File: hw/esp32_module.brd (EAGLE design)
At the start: 61.6 x 53.3 mm, 2 parts, among them IC1 ESP32-S2_WROVER, IC2 ESP32-WROVER

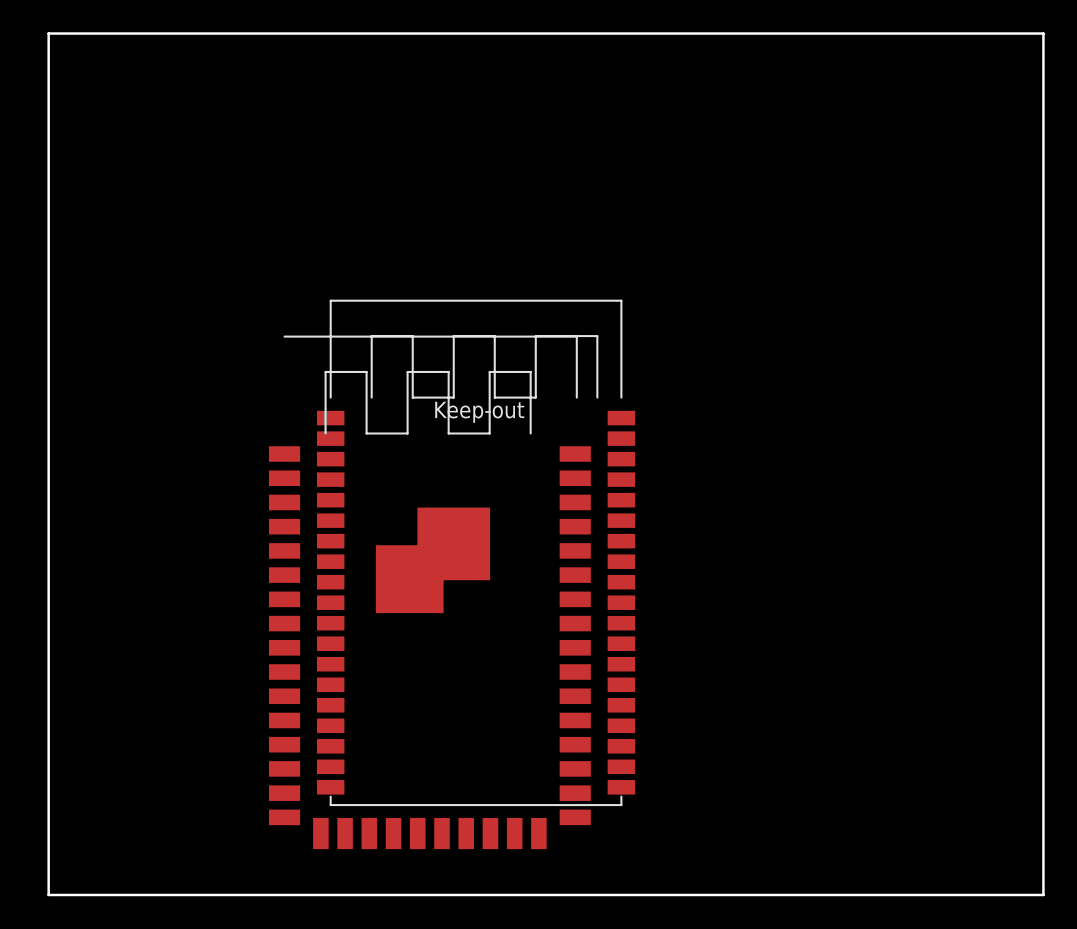
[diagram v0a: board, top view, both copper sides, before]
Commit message: improved
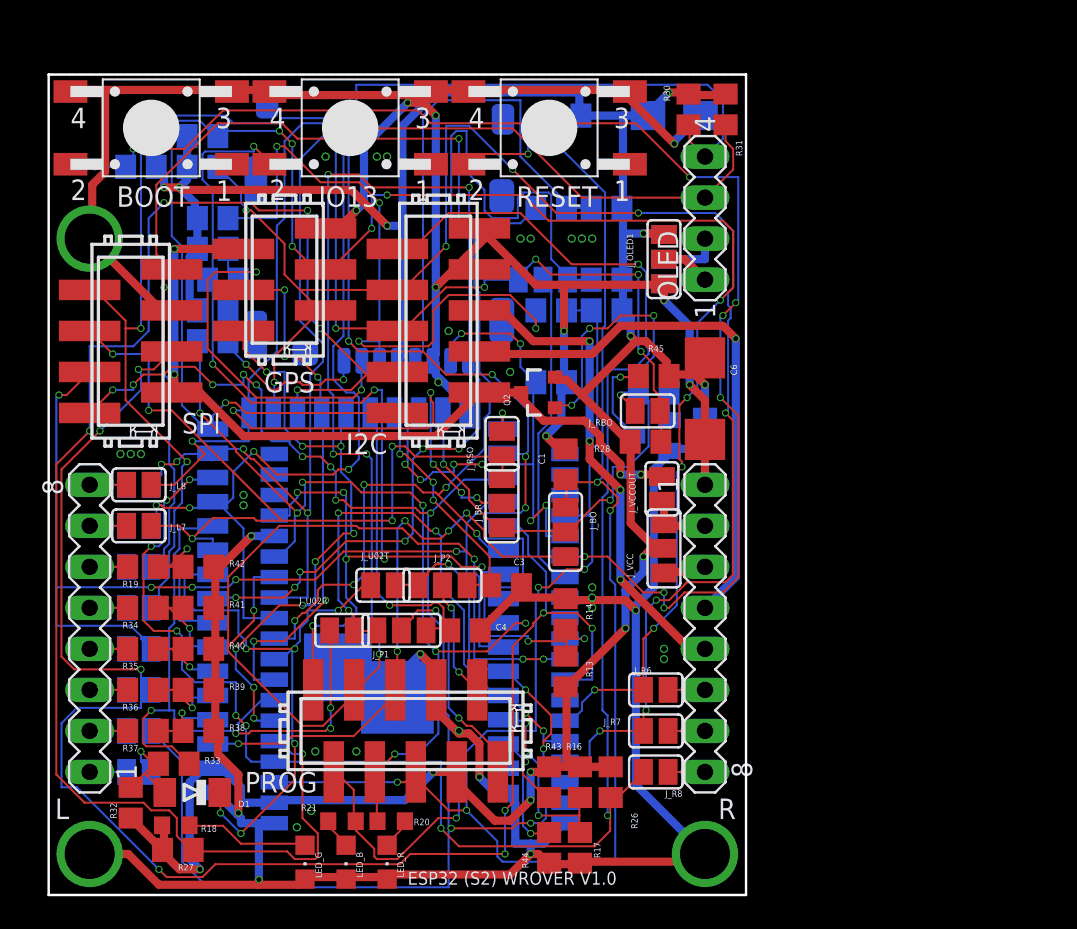
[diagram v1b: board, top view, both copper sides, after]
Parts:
- added BOOT, IO13, RESET: (no value), Ergaenzung:TASTER-9314_SMD
- added C1, C2: 0.1, rcl:C0805
- added C3, C4: 22p, rcl:C0805
- added C5: 10u, rcl:B/3528-21W
- added C6: (no value), rcl:C/6032-28R
- added D1: 4148, diode:MINIMELF
- added GPS: GPS, con-amp-micromatch:MICROMATCH-6SMD
- added I2C, PROG: I2CBUS, con-amp-micromatch:MICROMATCH-10SMD
- added J_BO, J_BR, J_IO4, J_OLED1, J_OLED2, J_P1, J_P2, J_VCC: (no value), jumper:SJ_2
- added J_L1, J_L2, J_L3, J_L4, J_L5, J_L6, J_L7, J_L7B, J_L8, J_L8B, J_R6, J_R7, J_R8, J_RBO, J_RSO, J_U02R, J_U02T, J_VCCOUT: (no value), jumper:SJ
- added L, R: (no value), con-lstb:MA08-1
- added LED_B, LED_G: G, led:CHIPLED_0805
- added LED_R: R, led:CHIPLED_0805
- added OLED: (no value), con-lstb:MA04-1
- added Q2: IRLML2244, User-Submitted:SOT23-3
- added R1, R15, R19, R2, R25, R26, R27, R28, R29, R3, R30, R31, R32, R33, R34, R35, R36, R37, R38, R39, R4, R40, R41, R42, R5, R6, R7, R8, R9: (no value), rcl:R0805
- added R10, R11, R12, R13, R14, R16, R17, R23, R43, R44, R45: 10k, rcl:R0805
- added R18, R20, R21: (no value), rcl:R0603
- added SDCARD: MICROSD_SD_MODE, con-molex-microsd:MICRO_SD_CONNECTOR
- added SPI: SPIBUS, con-amp-micromatch:MICROMATCH-8-SMD
- added T2: (no value), transistor:SOT23-BEC
- moved IC2 23.4 mm to (14.0, 28.6), flipped to the bottom, turned to 180 degrees
- moved IC1 21.4 mm to (10.2, 6.35), flipped to the bottom, turned to 180 degrees
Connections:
- new net BOOT: BOOT.2, IC1.3, IC2.IO0, J_BO.1, PROG.6, R11.1
- new net BUS_FON: I2C.3, IC1.19, IC2.SENSOR_VN, R27.2
- new net BUS_INT: I2C.9, IC1.14, IC2.SENSOR_VP, J_R8.2, R26.2
- new net BUS_ON: IC1.25, J_BO.2, J_BR.1, J_RBO.2, R23.1
- new net BUS_RESET: I2C.5, IC1.17, J_BR.2, J_IO4.3, J_L8.1, J_RBO.1, R28.2
- new net BUS_SCL: GPS.2, I2C.7, IC1.18, IC2.IO22, J_R7.2, R29.2
- new net BUS_SDA: GPS.4, I2C.1, IC1.16, IC2.IO21, J_R6.2, R25.2
- new net EN: C1.1, IC1.41, IC2.EN, J_BO.3, PROG.5, R10.1, RESET.2
- new net LCD_1: J_OLED1.2, OLED.1
- new net LCD_2: J_OLED2.2, OLED.2
- new net MTCK: IC1.33, IC2.IO13, IO13.2, PROG.10, R1.2
- new net MTDI: IC1.35, IC2.IO12, PROG.7, R15.2, R20.2
- new net MTDO: IC1.34, IC2.IO15, PROG.9, R12.1, R2.2, R21.2
- new net MTMS: IC1.36, IC2.IO14, PROG.8, R3.2
- new net N$1: IC2.IO4, J_IO4.2
- new net N$12: J_R8.1, R.8
- new net N$18: R23.2, T2.B
- new net N$2: Q2.1, R45.2, T2.C
- new net N$20: LED_R.A, R20.1
- new net N$21: LED_B.A, R21.1
- new net N$24: J_L7.2, J_L7B.2, L.7
- new net N$25: J_L6.2, L.6, R19.1
- new net N$27: J_L8.2, J_L8B.2, L.8
- new net N$28: J_L5.2, L.5, R34.1
- new net N$29: J_L4.2, L.4, R35.1
- new net N$3: J_R6.1, R.6
- new net N$30: J_L2.2, L.2, R37.1
- new net N$31: J_L3.2, L.3, R36.1
- new net N$32: J_L1.2, L.1
- new net N$34: J_P2.2, PROG.2
- new net N$4: LED_G.A, R18.1
- new net N$5: J_R7.1, R.7
- new net N$6: J_P1.2, PROG.1
- new net OLED_SCL: IC1.15, IC2.IO27, J_L8B.1, OLED.3, R31.2
- new net OLED_SDA: IC1.13, IC2.IO26, J_L7B.1, OLED.4, R30.2
- new net S2_IO1: IC1.4, R37.2, R38.1
- new net S2_IO2: IC1.5, R36.2, R39.1
- new net S2_IO3: IC1.6, R35.2, R40.1
- new net S2_IO4: IC1.7, R34.2, R41.1
- new net S2_IO45: IC1.39, R16.1, R17.2
- new net S2_IO46: IC1.40, R43.1, R44.2
- new net S2_IO5: IC1.8, R19.2, R42.1
- new net SD_CLK: R3.1, R6.2, SDCARD.5
- new net SD_CMD: R2.1, R7.2, SDCARD.3
- new net SD_D0: IC1.24, IC2.IO2, R4.2, SDCARD.7
- new net SD_D1: IC1.9, J_IO4.1, R5.2, SDCARD.8
- new net SD_D2: R15.1, R9.2, SDCARD.1
- new net SD_D3: R1.1, R8.2, SDCARD.2
- new net SPI_CS0: IC1.28, IC2.IO5, J_L5.1, R13.1, R14.2, SPI.7
- new net SPI_CS1: IC1.32, IC2.IO25, J_L6.1, SPI.8
- new net SPI_MISO: IC1.29, IC2.IO23, J_L2.1, SPI.1
- new net SPI_MOSI: IC1.31, IC2.IO19, J_L3.1, SPI.4
- new net SPI_ON: IC1.27, J_RSO.2
- new net SPI_RESET: IC1.11, J_BR.3, J_L7.1, J_RSO.1, SPI.5
- new net SPI_SCK: IC1.30, IC2.IO18, J_L4.1, SPI.3
- new net U0RXD: IC1.38, IC2.RXD0, J_P1.3, J_U02R.1
- new net U0TXD: IC1.37, IC2.TXD0, J_P2.3, J_U02T.1
- new net U1RXD: GPS.1, IC1.21, IC2.IO34
- new net U1TXD: GPS.3, IC1.20, IC2.IO32
- new net U2RXD: IC1.12, IC2.IO35, J_U02R.2, R33.2
- new net U2TXD: D1.C, IC1.10, IC2.IO33, J_U02T.2
- new net U2_BUS: D1.A, J_L1.1, R32.1, R33.1
- new net U33A: J_VCC.3, J_VCCOUT.2, R.2
- new net U33B: J_VCC.1, R.3
- new net U5: I2C.4, R.4
- new net UBAT: I2C.6, R.5
- new net UBUS: GPS.5, I2C.2, J_VCCOUT.1, Q2.3, SPI.2
- new net USBN: C4.1, IC1.22, J_P1.1
- new net USBP: C3.1, IC1.23, J_P2.1
- new net VCC: C2.1, C5.+, C6.+, IC1.2, IC2.VDD33, J_OLED1.3, J_OLED2.3, J_VCC.2, PROG.3, Q2.2, R10.2, R11.2, R12.2, R13.2, R16.2, R18.2, R25.1, R26.1, R27.1, R28.1, R29.1, R30.1, R31.1, R32.2, R43.2, R45.1, R5.1, R6.1, R7.1, R8.1, R9.1, SDCARD.4
- net GND: now also BOOT.3, BOOT.4, C1.2, C2.2, C3.2, C4.2, C5.-, C6.-, GPS.6, I2C.10, I2C.8, IC1.43, IC2.GND2, IO13.3, IO13.4, J_OLED1.1, J_OLED2.1, LED_B.C, LED_G.C, LED_R.C, PROG.4, R.1, R14.1, R17.1, R38.2, R39.2, R4.1, R40.2, R41.2, R42.2, R44.1, RESET.3, RESET.4, SDCARD.6, SPI.6, T2.E
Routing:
- net GND: track 0.00 -> 280.0 mm, vias 0 -> 45
- net VCC: track 0.00 -> 176.9 mm, vias 0 -> 13
- net BOOT: track 0.00 -> 121.4 mm, vias 0 -> 14
- net BUS_SDA: track 0.00 -> 116.8 mm, vias 0 -> 11
- net BUS_INT: track 0.00 -> 111.6 mm, vias 0 -> 9
- net SPI_CS0: track 0.00 -> 109.4 mm, vias 0 -> 8
- net BUS_RESET: track 0.00 -> 103.8 mm, vias 0 -> 11
- net SPI_MOSI: track 0.00 -> 101.9 mm, vias 0 -> 8
- net BUS_SCL: track 0.00 -> 100.3 mm, vias 0 -> 9
- net MTMS: track 0.00 -> 97.0 mm, vias 0 -> 7
- net BUS_FON: track 0.00 -> 96.6 mm, vias 0 -> 6
- net SPI_CS1: track 0.00 -> 94.2 mm, vias 0 -> 7
- net SPI_MISO: track 0.00 -> 93.4 mm, vias 0 -> 11
- net EN: track 0.00 -> 88.9 mm, vias 0 -> 5
- net OLED_SDA: track 0.00 -> 82.1 mm, vias 0 -> 6
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- added copper zone on layer 1, net GND
- added copper zone on layer 16, net GND
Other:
- board size 61.6 x 53.3 mm -> 43.2 x 50.8 mm
- board text added: "BOOT"
- board text added: "C1"
- board text added: "C2"
- board text added: "C3"
- board text added: "C4"
- board text added: "C5"
- board text added: "C6"
- board text added: "D1"
- board text added: "ESP32 (S2) WROVER V1.0"
- board text added: "GPS"
- board text added: "I2C"
- board text added: "IO13"
- board text added: "J_BO"
- board text added: "J_BR"
- board text added: "J_IO4"
- board text added: "J_L1"
- board text added: "J_L2"
- board text added: "J_L3"
- board text added: "J_L4"
- board text added: "J_L5"
- board text added: "J_L6"
- board text added: "J_L7"
- board text added: "J_L7B"
- board text added: "J_L8"
- board text added: "J_L8B"
- board text added: "J_OLED1"
- board text added: "J_OLED2"
- board text added: "J_P1"
- board text added: "J_P2"
- board text added: "J_R6"
- board text added: "J_R7"
- board text added: "J_R8"
- board text added: "J_RBO"
- board text added: "J_RSO"
- board text added: "J_U02R"
- board text added: "J_U02T"
- board text added: "J_VCC"
- board text added: "J_VCCOUT"
- board text added: "L"
- board text added: "LED_B"
- board text added: "LED_G"
- board text added: "LED_R"
- board text added: "OLED"
- board text added: "PROG"
- board text added: "Q2"
- board text added: "R"
- board text added: "R1"
- board text added: "R10"
- board text added: "R11"
- board text added: "R12"
- board text added: "R13"
- board text added: "R14"
- board text added: "R15"
- board text added: "R16"
- board text added: "R17"
- board text added: "R18"
- board text added: "R19"
- board text added: "R2"
- board text added: "R20"
- board text added: "R21"
- board text added: "R23"
- board text added: "R25"
- board text added: "R26"
- board text added: "R27"
- board text added: "R28"
- board text added: "R29"
- board text added: "R3"
- board text added: "R30"
- board text added: "R31"
- board text added: "R32"
- board text added: "R33"
- board text added: "R34"
- board text added: "R35"
- board text added: "R36"
- board text added: "R37"
- board text added: "R38"
- board text added: "R39"
- board text added: "R4"
- board text added: "R40"
- board text added: "R41"
- board text added: "R42"
- board text added: "R43"
- board text added: "R44"
- board text added: "R45"
- board text added: "R5"
- board text added: "R6"
- board text added: "R7"
- board text added: "R8"
- board text added: "R9"
- board text added: "RESET"
- board text added: "SDCARD"
- board text added: "SPI"
- board text added: "T2"
